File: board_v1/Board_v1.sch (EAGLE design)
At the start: 19 parts, among them IC1 MAX7219, IC2 MAX7219, IC3 MAX7219

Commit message: PCB v1 WIP
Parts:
- removed U$1: MRB_ROTARY_SWITCH, AES_lib:MRB_ROTARY_SWITCH
- added 12VIN: CONN3, AES_lib:MICRO-FIT_3.0_43650
- added BTN: CONN1, AES_lib:MICRO-FIT_3.0_43650
- added C1, C2, C3: 10uF, AES_lib:CAP_POL
- added C4, C5, C6: 100nF, AES_lib:CAP_CERAMIC
- added D1: 1N4001, AES_lib:1N4001
- added MOSFET: IRLB872, AES_lib:IRLB872
- added R1: 28k, AES_lib:RESISTOR
- added R2, R3: 23k, AES_lib:RESISTOR
- added R4: 10k, AES_lib:RESISTOR
- added SOUT: CONN2, AES_lib:MICRO-FIT_3.0_43650
- added SW1: ROTARY SWITCH, AES_lib:MRB_ROTARY_SWITCH
- added VREG: L7805CV, AES_lib:L7805CV
- CONV: value 3-5V_LOGIC_LVL_CONV -> LOGIC LVL CONV
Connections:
- new net 12V: 12VIN.P$2, D1.C, SOUT.P$2, VREG.IN
- new net 3.3V: FEATHERM0.3V
- new net 5V: FEATHERM0.USB, IC1.VCC, IC2.VCC, IC3.VCC, R1.1, R2.1, R3.1, VREG.OUT
- new net GND: 12VIN.P$1, CONV.HGND, CONV.LGDN, FEATHERM0.GND, IC1.GND@1, IC1.GND@2, IC2.GND@1, IC2.GND@2, IC3.GND@1, IC3.GND@2, MOSFET.S, R4.1, VREG.GND
- new net N$1: IC1.ISET, R1.2
- new net N$10: IC1.CLK, IC2.CLK, IC3.CLK
- new net N$11: IC1.LOAD, IC2.LOAD, IC3.LOAD
- new net N$12: IC1.DIN
- new net N$13: IC1.DOUT, IC3.DIN
- new net N$14: IC2.DIN, IC3.DOUT
- new net N$2: D1.A, MOSFET.D, SOUT.P$1
- new net N$3: MOSFET.G
- new net N$4: SW1.1
- new net N$5: SW1.2
- new net N$6: SW1.3
- new net N$7: R4.2, SW1.C1
- new net N$8: IC2.ISET, R3.2
- new net N$9: IC3.ISET, R2.2
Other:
- note added: "to arduino pin"
- note added: "to arduino pin (via level converter)"
- moved on the sheet: BAR1, BAR2, BAR3, CONV, IC1, IC2, IC3, SEV1, SEV10, SEV2, SEV3, SEV4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

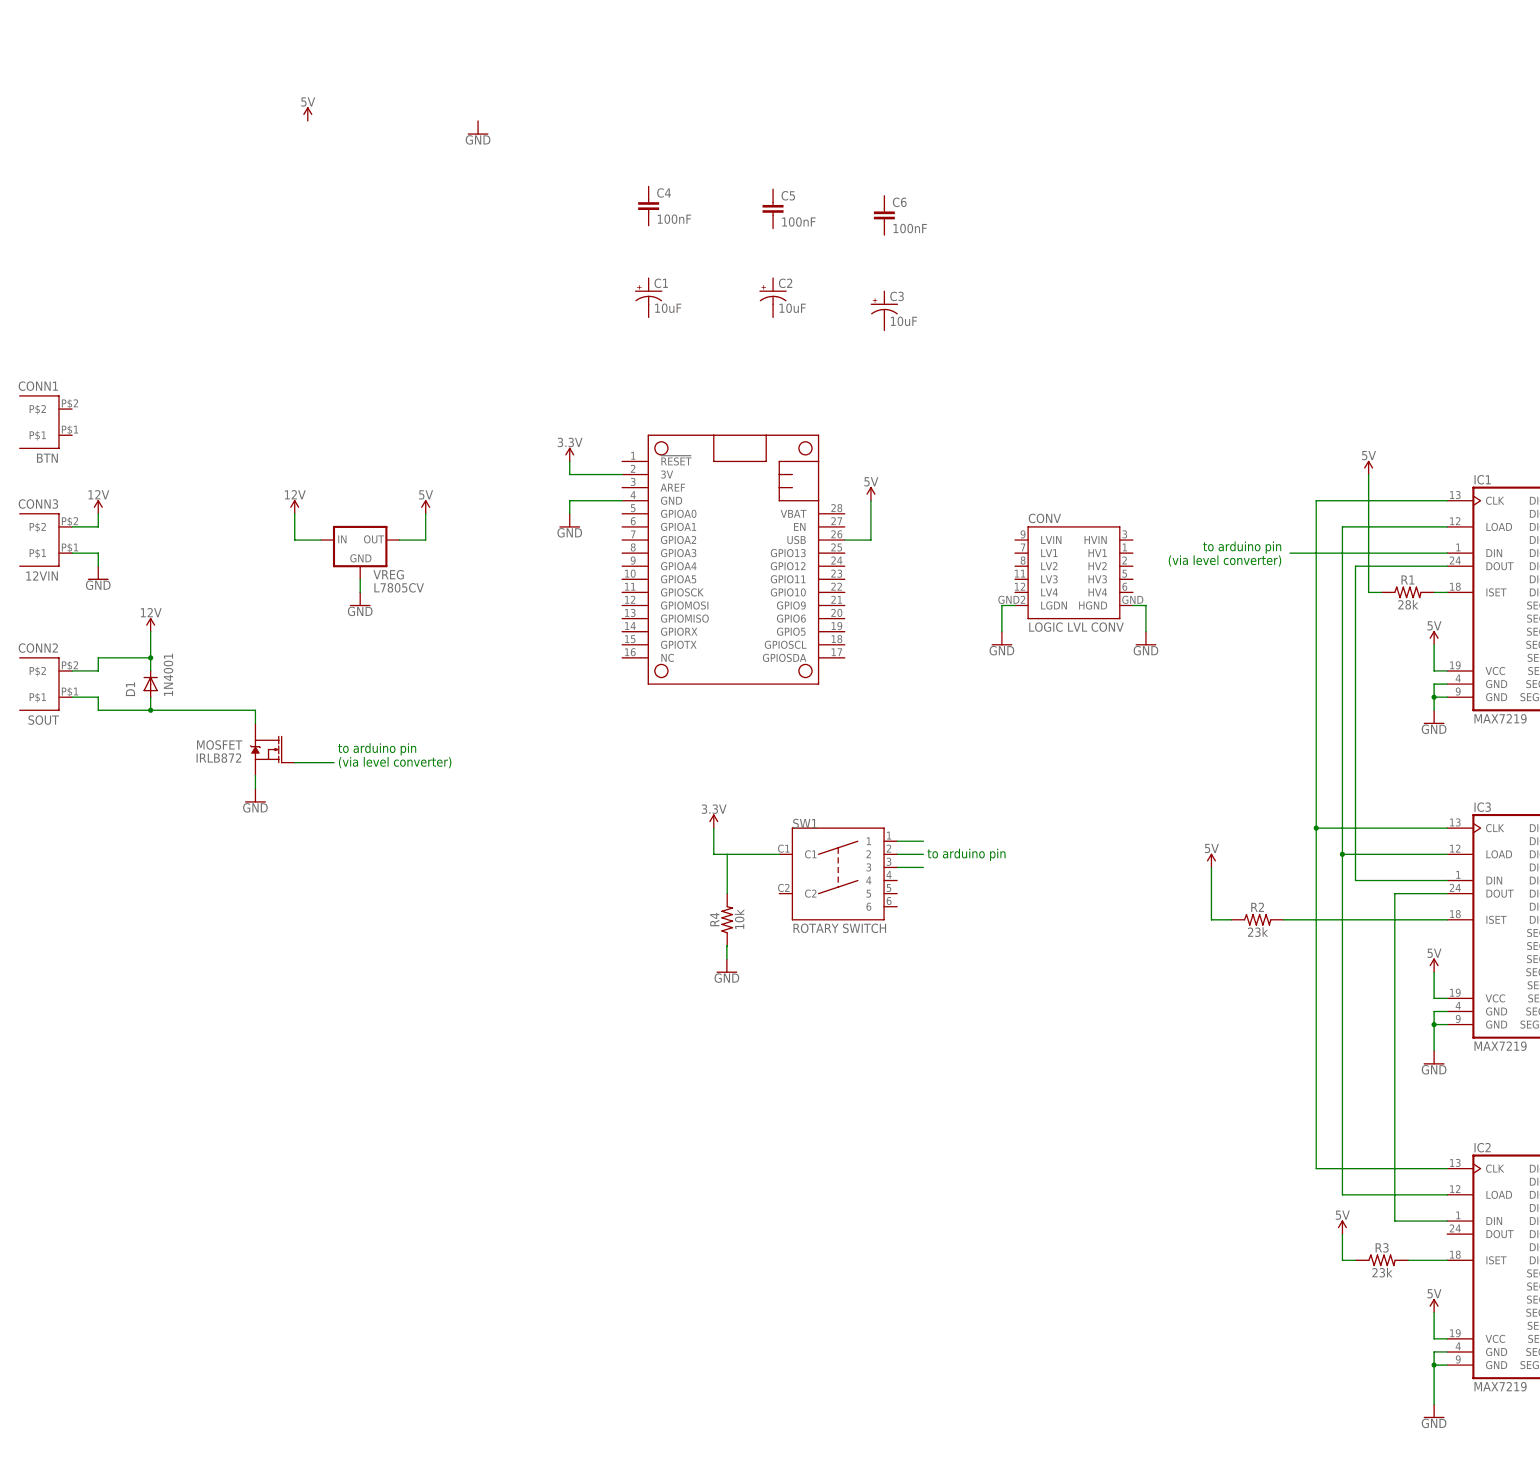
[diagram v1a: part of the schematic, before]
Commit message: added button pcb
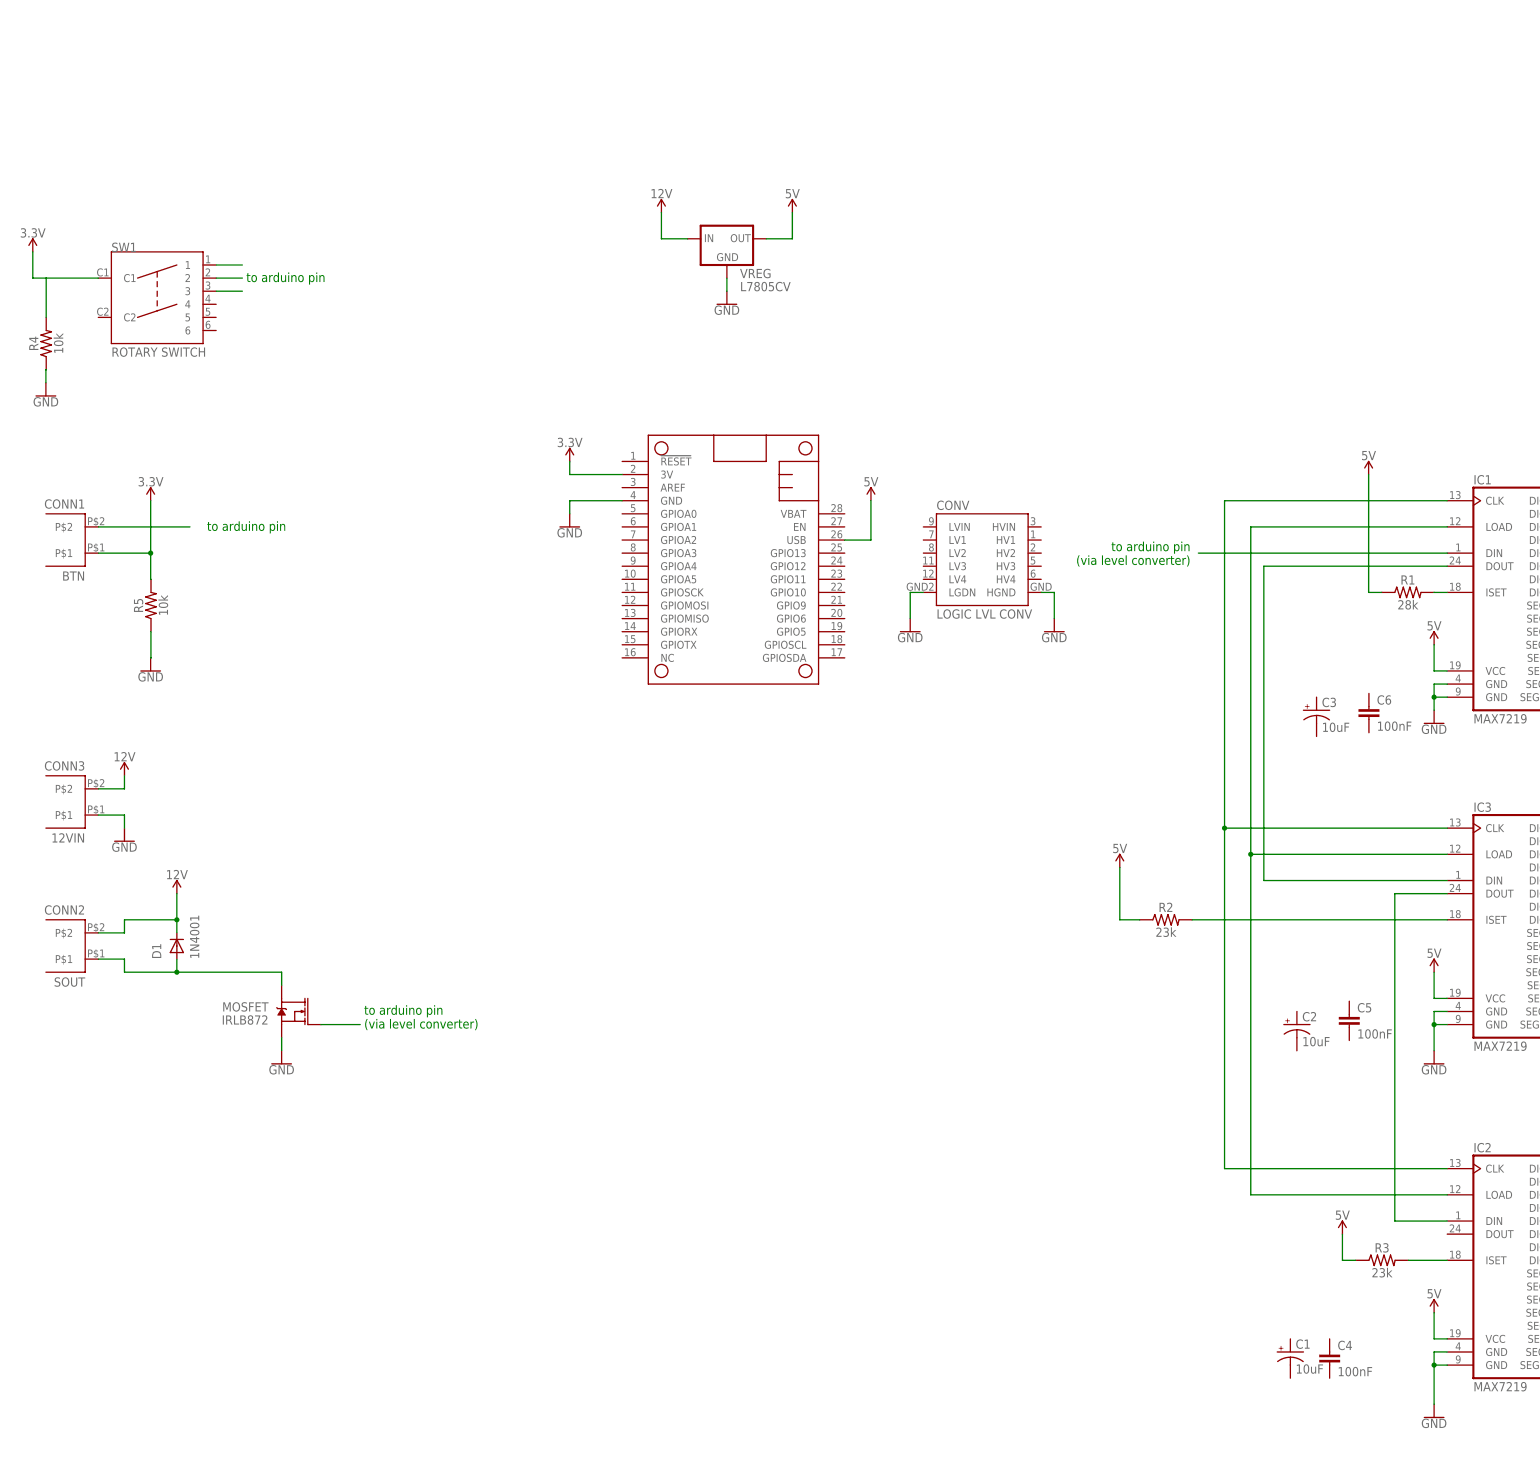
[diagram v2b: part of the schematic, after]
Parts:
- added R5: 10k, AES_lib:RESISTOR
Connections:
- new net N$16: BTN.P$2
- net 3.3V: now also BTN.P$1, R5.2
- net GND: now also R5.1
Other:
- moved on the sheet: 12VIN, BTN, C1, C2, C3, C4, C5, C6, CONV, D1, MOSFET, R2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

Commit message: ready to start routing?
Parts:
- added J1: (no value), SparkFun-Connectors:CONN_041X04_NO_SILK
- added R6: 10k, AES_lib:RESISTOR
- C2: value 10uF -> 100nF; device AES_lib:CAP_POL -> AES_lib:CAP_CERAMIC
- C5: value 100nF -> 10uF; device AES_lib:CAP_CERAMIC -> AES_lib:CAP_POL
- R2: value 23k -> 28k
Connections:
- removed net N$10: IC1.CLK, IC2.CLK, IC3.CLK
- removed net N$11: IC1.LOAD, IC2.LOAD, IC3.LOAD
- removed net N$12: IC1.DIN
- removed net N$16: BTN.P$2
- removed net N$4: SW1.1
- removed net N$5: SW1.2
- removed net N$6: SW1.3
- new net BTN: BTN.P$2, FEATHERM0.GPIO9
- new net CLK: CONV.HV1, IC1.CLK, IC2.CLK, IC3.CLK
- new net CLK3: CONV.LV1, FEATHERM0.GPIO12
- new net DIG01: BAR2.C0, IC1.DIG0
- new net DIG02: BAR1.C0, IC2.DIG0
- new net DIG03: IC3.DIG0, SEV7.1-6C
- new net DIG11: BAR2.C1, IC1.DIG1
- new net DIG12: BAR1.C1, IC2.DIG1
- new net DIG13: IC3.DIG1, SEV8.1-6C
- new net DIG21: BAR2.C2, IC1.DIG2
- new net DIG22: BAR1.C2, IC2.DIG2
- new net DIG23: IC3.DIG2, SEV9.1-6C
- new net DIG31: BAR3.C0, IC1.DIG3
- new net DIG32: IC2.DIG3, SEV1.1-6C
- new net DIG33: IC3.DIG3, SEV10.1-6C
- new net DIG41: BAR3.C1, IC1.DIG4
- new net DIG42: IC2.DIG4, SEV2.1-6C
- new net DIG43: IC3.DIG4, SEV5.1-6C
- new net DIG51: BAR3.C2, IC1.DIG5
- new net DIG52: IC2.DIG5, SEV3.1-6C
- new net DIG53: IC3.DIG5, SEV6.1-6C
- new net DIG62: IC2.DIG6, SEV4.1-6C
- new net DIN: CONV.HV3, IC1.DIN
- new net DIN3: CONV.LV3, FEATHERM0.GPIO10
- new net LOAD: CONV.HV2, IC1.LOAD, IC2.LOAD, IC3.LOAD
- new net LOAD3: CONV.LV2, FEATHERM0.GPIO11
- new net RESET: FEATHERM0.!RESET, J1.2
- new net S1: FEATHERM0.GPIO6, SW1.1
- new net S2: FEATHERM0.GPIO5, SW1.2
- new net S3: FEATHERM0.GPIOSCL, SW1.3
- new net SEGA1: BAR2.A1, BAR3.A1, IC1.SEGA
- new net SEGA2: BAR1.A1, IC2.SEGA, SEV1.10A, SEV2.10A, SEV3.10A, SEV4.10A
- new net SEGA3: IC3.SEGA, SEV10.10A, SEV5.10A, SEV6.10A, SEV7.10A, SEV8.10A, SEV9.10A
- new net SEGB1: BAR2.A2, BAR3.A2, IC1.SEGB
- new net SEGB2: BAR1.A2, IC2.SEGB, SEV1.9B, SEV2.9B, SEV3.9B, SEV4.9B
- new net SEGB3: IC3.SEGB, SEV10.9B, SEV5.9B, SEV6.9B, SEV7.9B, SEV8.9B, SEV9.9B
- new net SEGC1: BAR2.A3, BAR3.A3, IC1.SEGC
- new net SEGC2: BAR1.A3, IC2.SEGC, SEV1.8C, SEV2.8C, SEV3.8C, SEV4.8C
- new net SEGC3: IC3.SEGC, SEV10.8C, SEV5.8C, SEV6.8C, SEV7.8C, SEV8.8C, SEV9.8C
- new net SEGD1: BAR2.A4, BAR3.A4, IC1.SEGD
- new net SEGD2: BAR1.A4, IC2.SEGD, SEV1.5D, SEV2.5D, SEV3.5D, SEV4.5D
- new net SEGD3: IC3.SEGD, SEV10.5D, SEV5.5D, SEV6.5D, SEV7.5D, SEV8.5D, SEV9.5D
- new net SEGDP1: BAR2.A8, BAR3.A8, IC1.SEGDP
- new net SEGDP2: BAR1.A8, IC2.SEGDP, SEV1.7DP, SEV2.7DP, SEV3.7DP, SEV4.7DP
- new net SEGDP3: IC3.SEGDP, SEV10.7DP, SEV5.7DP, SEV6.7DP, SEV7.7DP, SEV8.7DP, SEV9.7DP
- new net SEGE1: BAR2.A5, BAR3.A5, IC1.SEGE
- new net SEGE2: BAR1.A5, IC2.SEGE, SEV1.4E, SEV2.4E, SEV3.4E, SEV4.4E
- new net SEGE3: IC3.SEGE, SEV10.4E, SEV5.4E, SEV6.4E, SEV7.4E, SEV8.4E, SEV9.4E
- new net SEGF1: BAR2.A6, BAR3.A6, IC1.SEGF
- new net SEGF2: BAR1.A6, IC2.SEGF, SEV1.2F, SEV2.2F, SEV3.2F, SEV4.2F
- new net SEGF3: IC3.SEGF, SEV10.2F, SEV5.2F, SEV6.2F, SEV7.2F, SEV8.2F, SEV9.2F
- new net SEGG1: BAR2.A7, BAR3.A7, IC1.SEGG
- new net SEGG2: BAR1.A7, IC2.SEGG, SEV1.3G, SEV2.3G, SEV3.3G, SEV4.3G
- new net SEGG3: IC3.SEGG, SEV10.3G, SEV5.3G, SEV6.3G, SEV7.3G, SEV8.3G, SEV9.3G
- new net STA: FEATHERM0.GPIOSDA, J1.3
- net 3.3V: now also CONV.LVIN, J1.4, R6.2
- net 5V: now also C1.+, C2.1, C3.+, C4.1, C5.+, C6.1, CONV.HVIN
- net GND: now also C1.-, C2.2, C3.-, C4.2, C5.-, C6.2, J1.1, R6.1
- net N$13: now also IC2.DIN; no longer IC3.DIN
- net N$14: now also IC2.DOUT, IC3.DIN; no longer IC2.DIN, IC3.DOUT
- net N$3: now also CONV.HV4
- net N$8: now also IC3.ISET; no longer IC2.ISET
- net N$9: now also IC2.ISET; no longer IC3.ISET
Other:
- note added: "n.c."
- note removed: "to arduino pin"
- note removed: "to arduino pin (via level converter)"
- moved on the sheet: 12VIN, BAR1, BAR2, BAR3, BTN, C1, C3, C4, C6, CONV, D1, IC1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
